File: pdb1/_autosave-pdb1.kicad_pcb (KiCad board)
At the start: 2 copper layers, 97.8 x 17.8 mm, 20 parts, among them P2 CONN_XT60, P3 CONN_02X03, P4 CONN_02X03, P5 CONN_01X03, P6 CONN_XT60, Q2 BUK9Y4R8-60E, U1 INA169, U2 NSI45020AT1G, U3 NSI45020AT1G, U7 MIC5014, U8 NSI45020AT1G

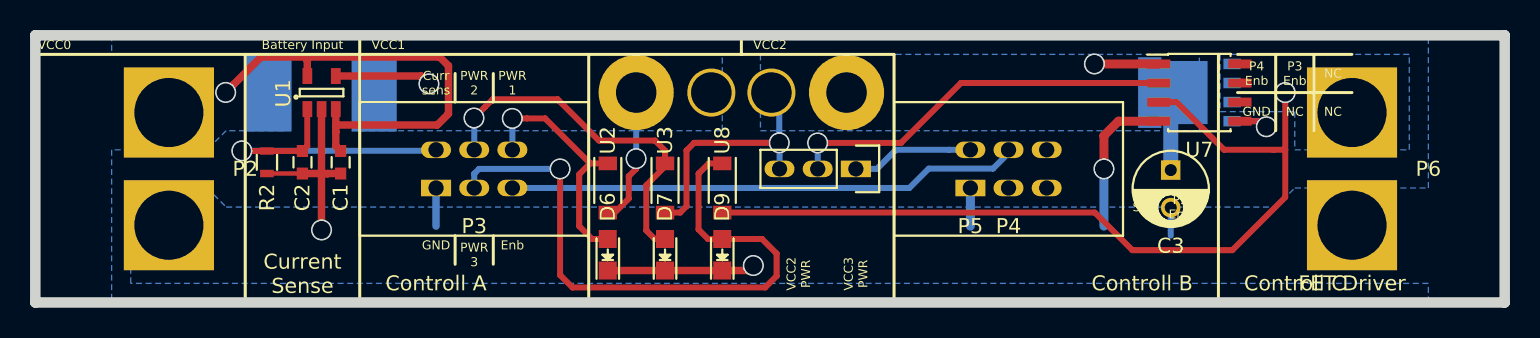
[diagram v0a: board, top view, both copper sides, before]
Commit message: test
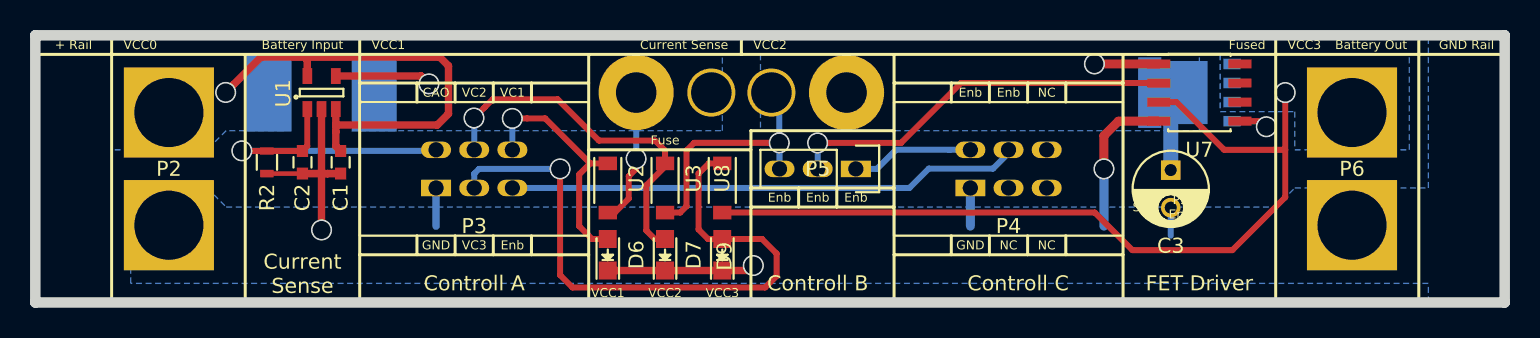
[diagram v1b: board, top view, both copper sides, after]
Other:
- board text added: "+ Rail"
- board text added: "Battery Out"
- board text added: "CAO"
- board text added: "Fuse"
- board text added: "Fused"
- board text added: "GND Rail"
- board text added: "VC1"
- board text added: "VC2"
- board text added: "VC3"
- board text added: "VCC3"
- board text removed: "Curr sens"
- board text removed: "P3 Enb"
- board text removed: "P4 Enb"
- board text removed: "PWR 1"
- board text removed: "PWR 2"
- board text removed: "PWR 3"
- board text removed: "VCC2 PWR"
- board text removed: "VCC3 PWR"
